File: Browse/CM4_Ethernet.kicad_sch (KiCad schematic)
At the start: 6 parts

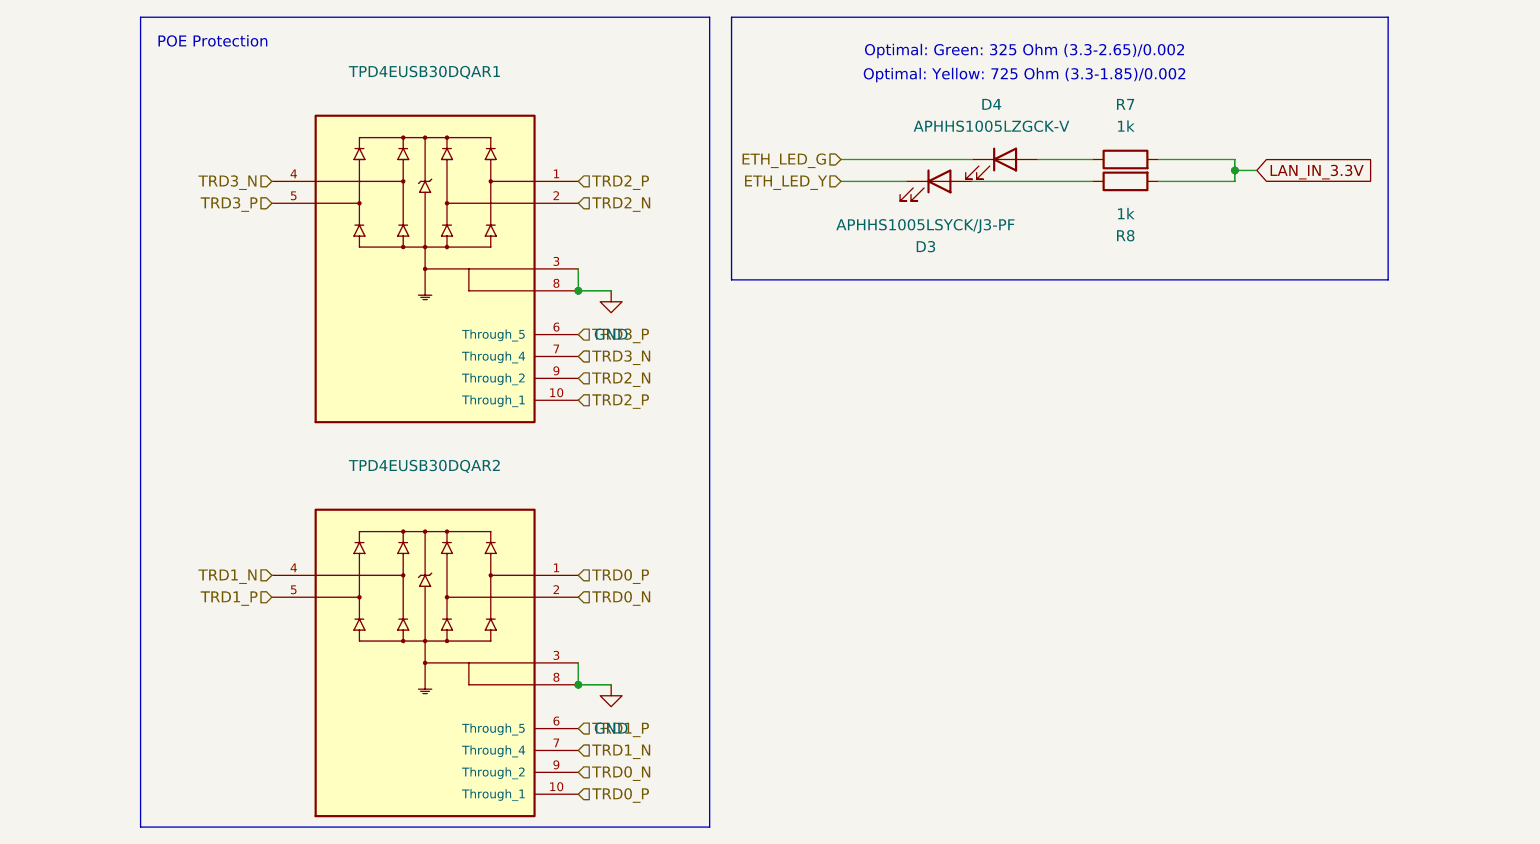
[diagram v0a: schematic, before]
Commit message: Deploying to gh-pages from @ Nautilus-UUV/nautilus-mainboard-PCB@b62834b88bb3e2a9413bcb4ea8e223af403e20ba 🚀
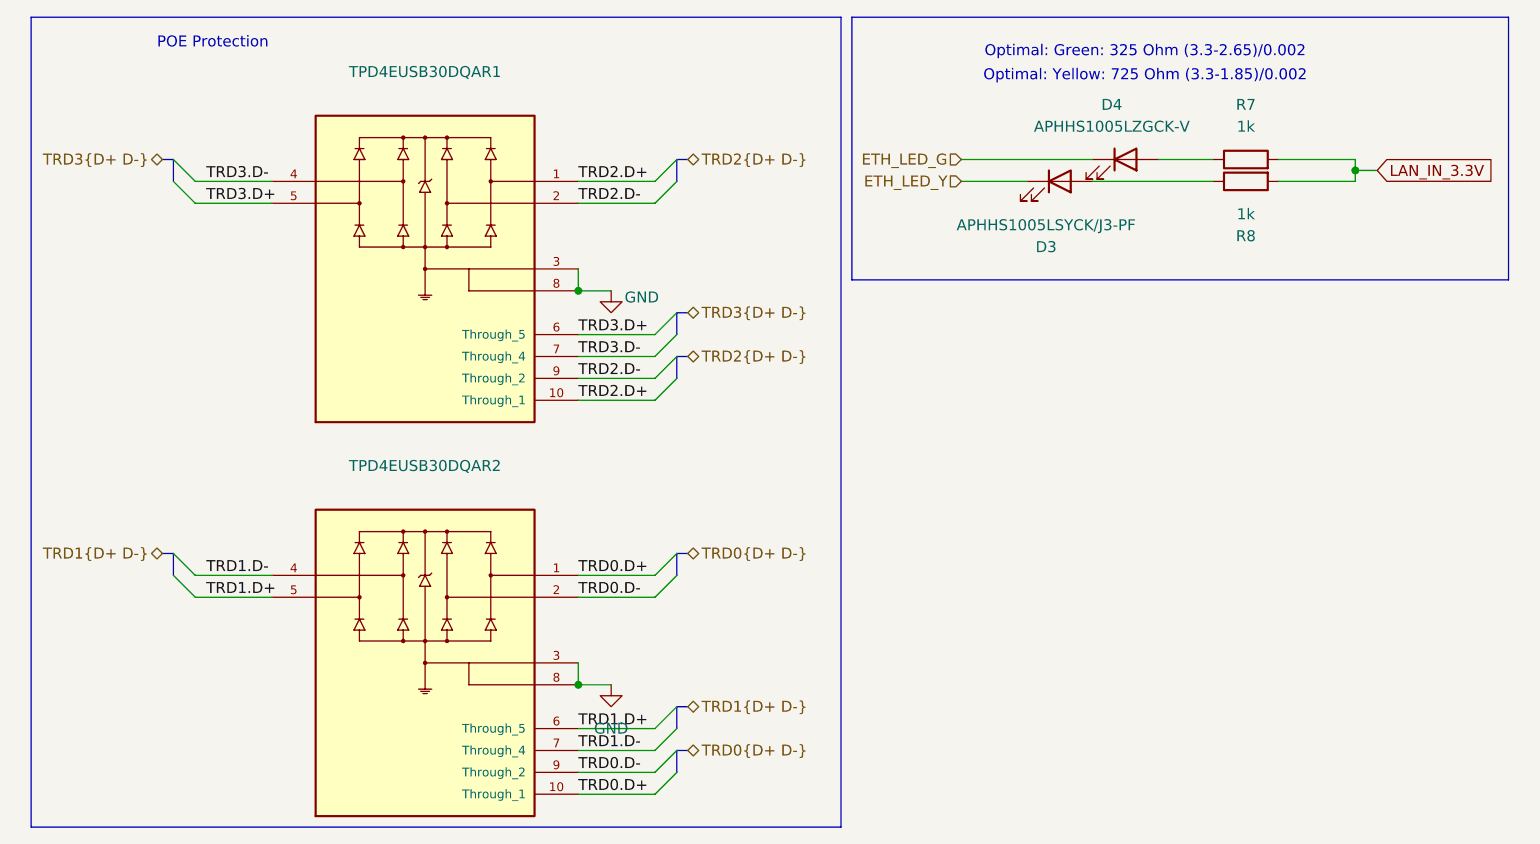
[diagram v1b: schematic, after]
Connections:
- net TRD0_N renamed TRD0.D-
- net TRD0_P renamed TRD0.D+
- net TRD1_N renamed TRD1.D-
- net TRD1_P renamed TRD1.D+
- net TRD2_N renamed TRD2.D-
- net TRD2_P renamed TRD2.D+
- net TRD3_N renamed TRD3.D-
- net TRD3_P renamed TRD3.D+
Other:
- moved on the sheet: D3, D4, R7, R8
